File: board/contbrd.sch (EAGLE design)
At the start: 35 parts, among them IC1 STM32F205RGT, IC2 74HCT244DW, IC3 74HCT244DW, IC4 LM3940, J1 DCJ0202

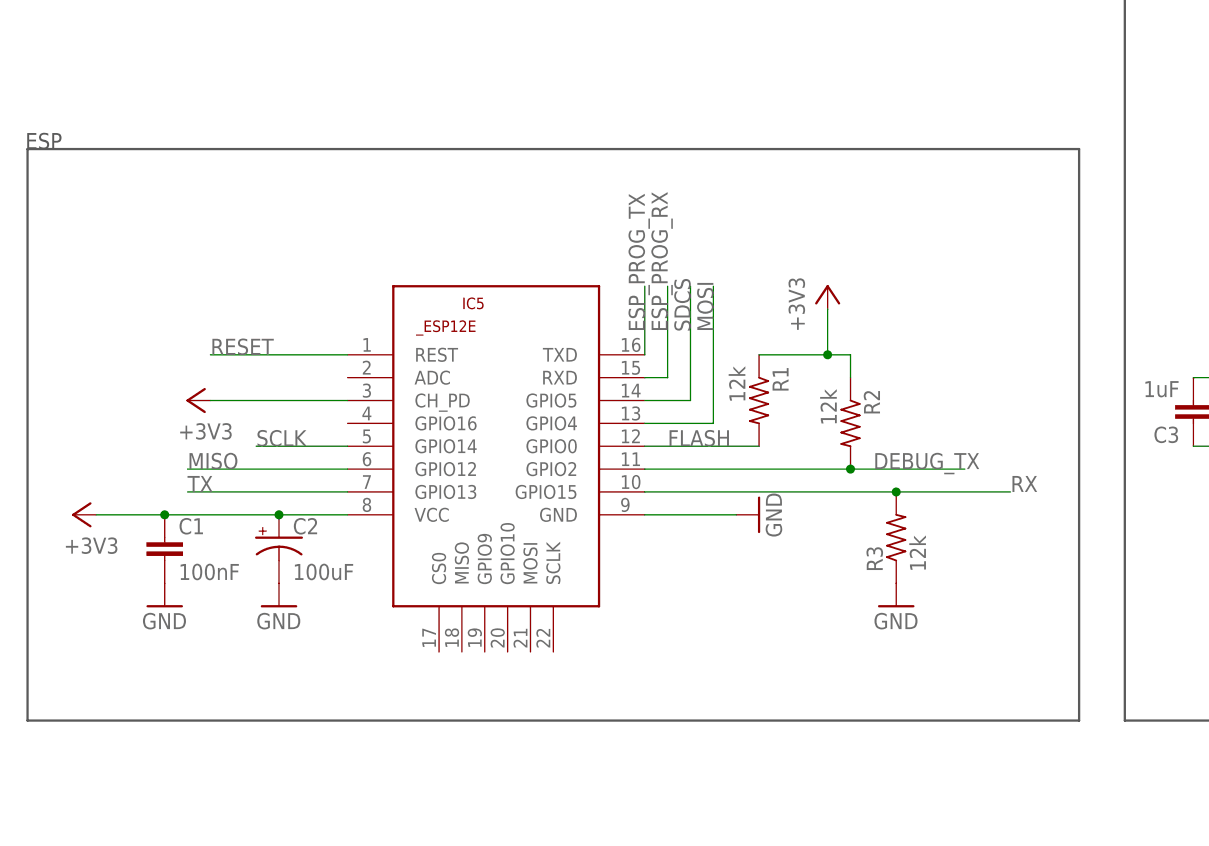
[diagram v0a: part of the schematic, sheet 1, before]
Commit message: board rev b final final
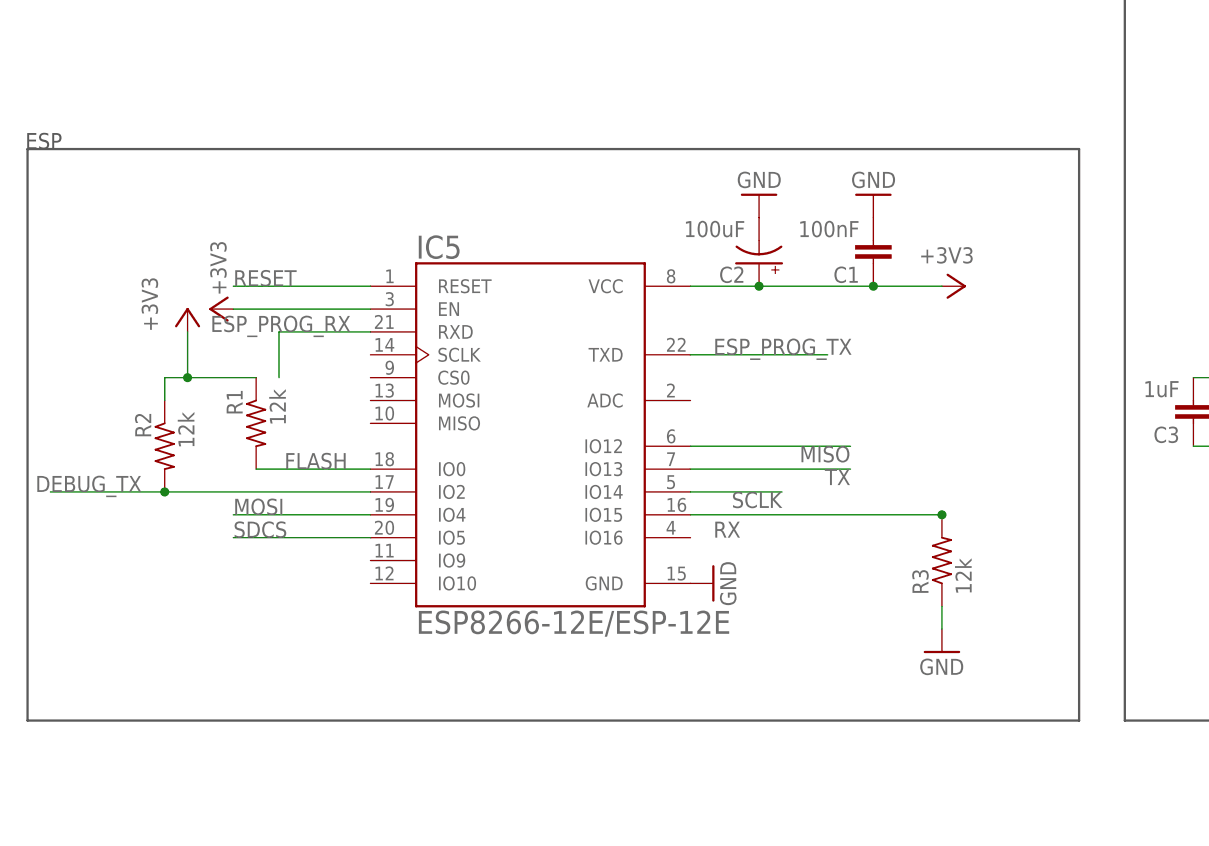
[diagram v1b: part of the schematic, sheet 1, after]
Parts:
- IC5: value (none) -> ESP8266-12E/ESP-12E; device esp12e:ESP8266-12EESP12E -> ESP8266-12E_ESP-12E:ESP8266-12E/ESP-12E
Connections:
- net +3V3: now also IC5.EN; no longer IC5.CH_PD
- net DEBUG_TX: now also IC5.IO2; no longer IC5.GPIO2
- net FLASH: now also IC5.IO0; no longer IC5.GPIO0
- net MISO: now also IC5.IO12; no longer IC5.GPIO12
- net MOSI: now also IC5.IO4; no longer IC5.GPIO4
- net RESET: now also IC5.RESET; no longer IC5.REST
- net RX: now also IC5.IO15; no longer IC5.GPIO15
- net SCLK: now also IC5.IO14; no longer IC5.GPIO14
- net SDCS: now also IC5.IO5; no longer IC5.GPIO5
- net TX: now also IC5.IO13; no longer IC5.GPIO13
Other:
- moved on the sheet: C1, C2, IC5, R1, R2, R3
